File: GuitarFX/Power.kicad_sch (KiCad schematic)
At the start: 20 parts, among them J201 Jack-DC, U3 NCP718xSN500, U4 NCP1117-3.3_SOT223

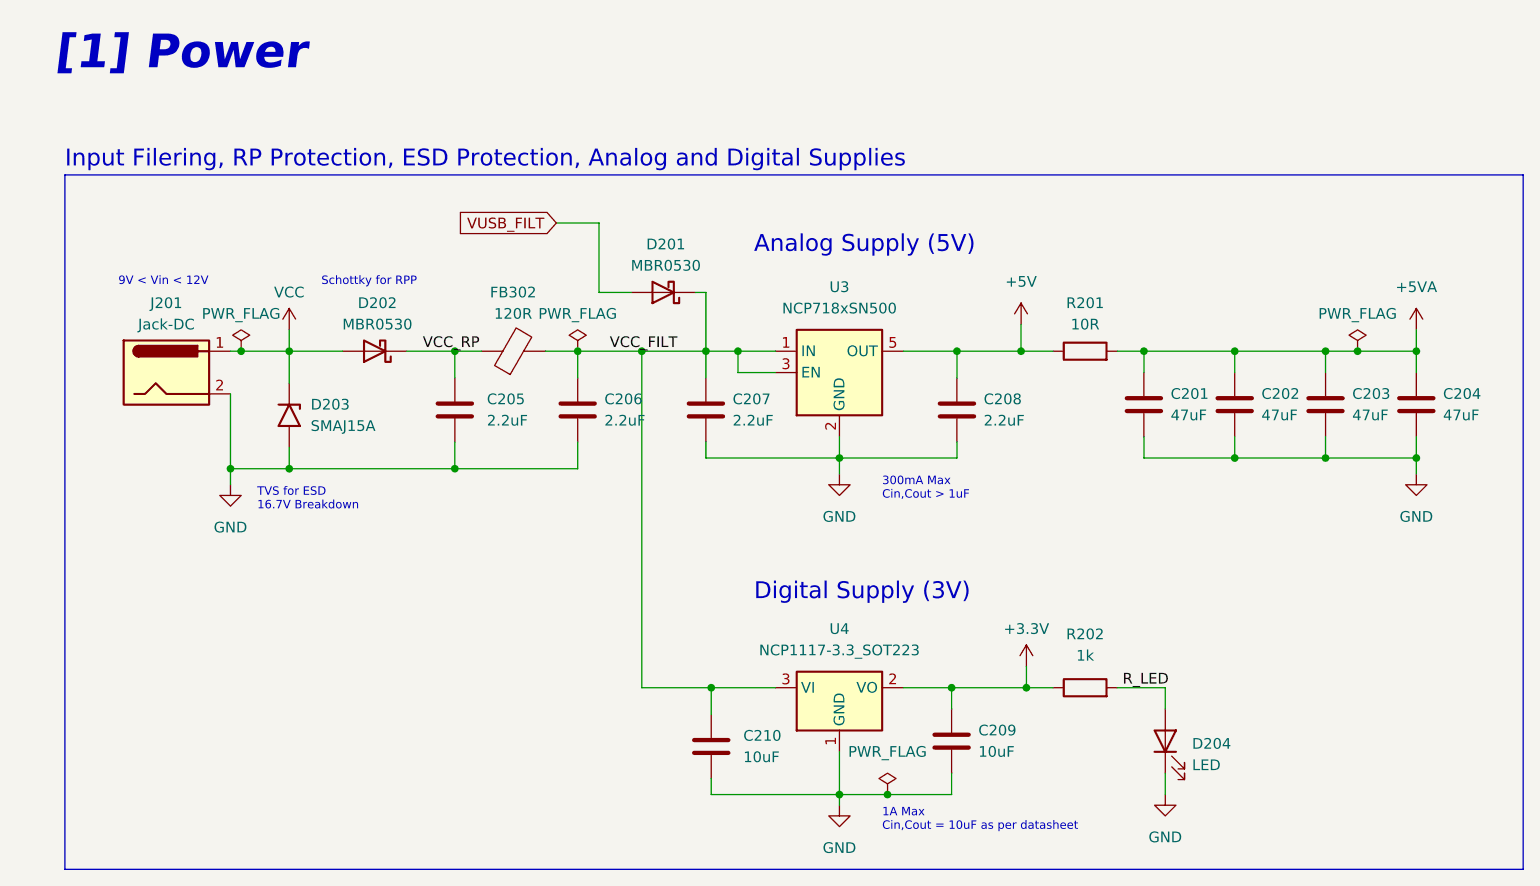
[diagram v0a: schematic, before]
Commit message: Assigned all footprints
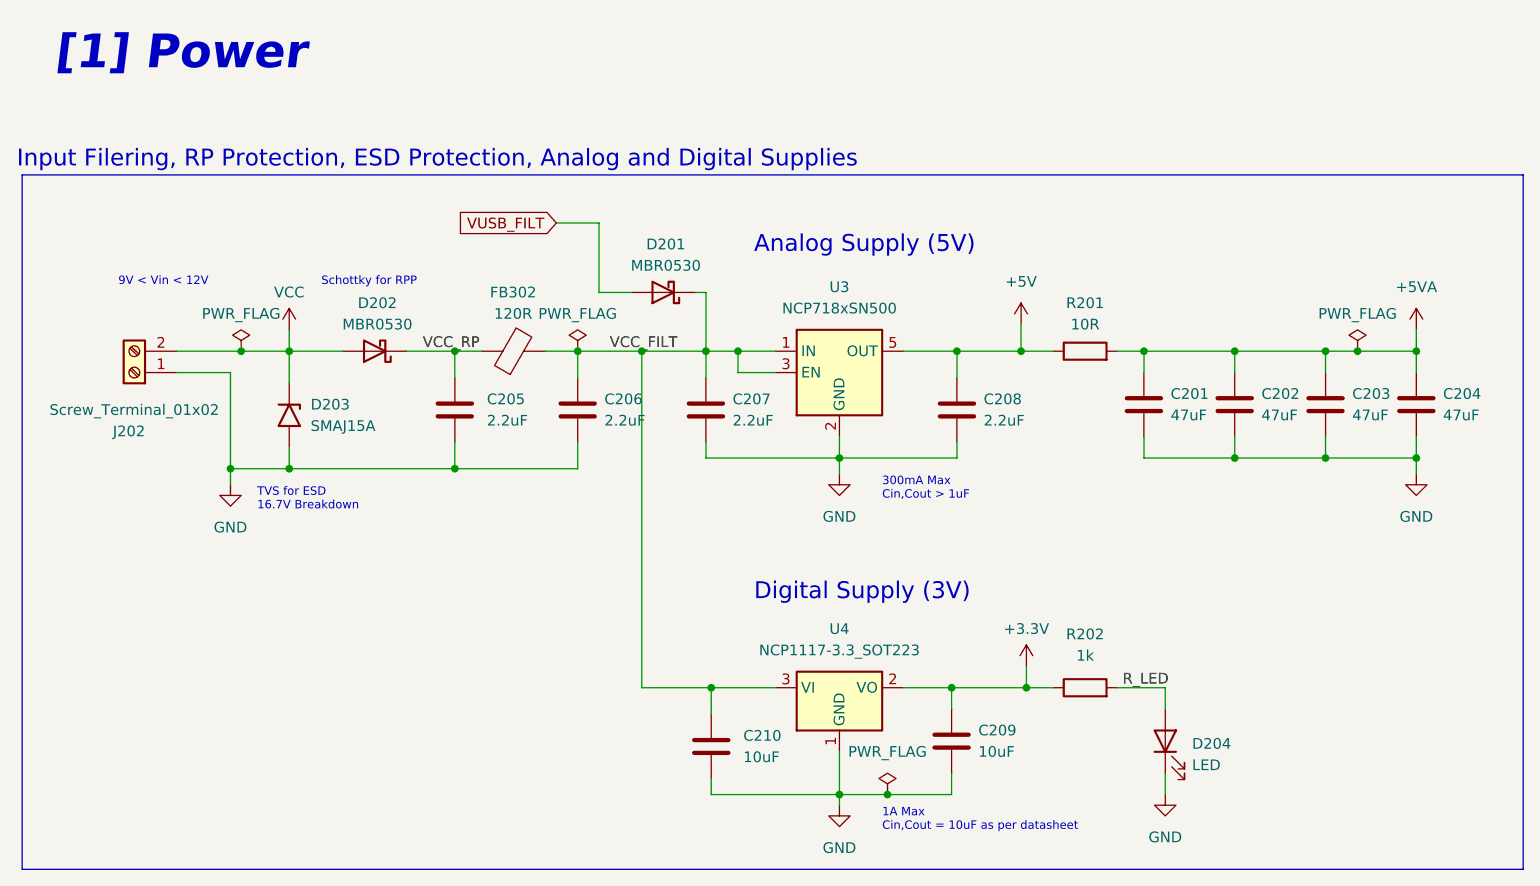
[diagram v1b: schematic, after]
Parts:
- removed J201: Jack-DC, symbol Connector:Jack-DC
- added J202: Screw_Terminal_01x02, TerminalBlock_Phoenix:TerminalBlock_Phoenix_MPT-0,5-2-2.54_1x02_P2.54mm_Horizontal, symbol Connector:Screw_Terminal_01x02
- FB302: footprint (none) -> Inductor_SMD:L_0603_1608Metric
- R201: footprint (none) -> TerminalBlock_Phoenix:TerminalBlock_Phoenix_MPT-0,5-6-2.54_1x06_P2.54mm_Horizontal
- R202: footprint (none) -> TerminalBlock_Phoenix:TerminalBlock_Phoenix_MPT-0,5-4-2.54_1x04_P2.54mm_Horizontal
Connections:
- net GND: now also J202.1 (Pin_1)
- net VCC: now also J202.2 (Pin_2)
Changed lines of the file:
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@@
-    (stroke (width 0) (type default))
-  )
-  (wire (pts (xy 60.96 62.865) (xy 62.23 62.865))
     (stroke (width 0) (type default))
   )
@@
     (stroke (width 0) (type default))
   )
+  (wire (pts (xy 54.61 62.865) (xy 62.23 62.865))
+    (stroke (width 0) (type default))
+  )
   (wire (pts (xy 118.11 115.57) (xy 133.35 115.57))
     (stroke (width 0) (type default))
@@
     (stroke (width 0) (type default))
   )
-  (wire (pts (xy 60.96 67.945) (xy 60.96 76.835))
+  (wire (pts (xy 60.96 65.405) (xy 60.96 76.835))
     (stroke (width 0) (type default))
   )
@@
     (stroke (width 0) (type default))
   )
+  (wire (pts (xy 54.61 65.405) (xy 60.96 65.405))
+    (stroke (width 0) (type default))
+  )
   (wire (pts (xy 191.135 73.025) (xy 191.135 75.565))
     (stroke (width 0) (type default))
@@
     (stroke (width 0) (type default))
   )
-  (rectangle (start 41.275 41.91) (end 214.63 124.46)
+  (rectangle (start 36.195 41.91) (end 214.63 124.46)
     (stroke (width 0) (type default))
     (fill (type none))
@@
   )
   (text "Input Filering, RP Protection, ESD Protection, Analog and Digital Supplies"
-    (at 41.275 41.275 0)
+    (at 35.56 41.275 0)
     (effects (font (size 2 2)) (justify left bottom))
   )
@@
       (effects (font (size 1.27 1.27)))
     )
-    (property "Footprint" "" (at 162.56 104.648 90)
+    (property "Footprint" "TerminalBlock_Phoenix:TerminalBlock_Phoenix_MPT-0,5-4-2.54_1x04_P2.54mm_Horizontal" (at 162.56 104.648 90)
       (effects (font (size 1.27 1.27)) hide)
     )
@@
       (effects (font (size 1.27 1.27)))
     )
-    (property "Footprint" "" (at 162.56 64.643 90)
+    (property "Footprint" "TerminalBlock_Phoenix:TerminalBlock_Phoenix_MPT-0,5-6-2.54_1x06_P2.54mm_Horizontal" (at 162.56 64.643 90)
       (effects (font (size 1.27 1.27)) hide)
     )
@@
         (path "/4ab4bfc6-98ca-4cb1-8273-436b96035b51/171d6b95-1f9c-4c9d-954a-bc461d0cb77a"
           (reference "R201") (unit 1)
-        )
-      )
-    )
-  )
-  (symbol (lib_id "Connector:Jack-DC") (at 53.34 65.405 0) (unit 1)
-    (in_bom yes) (on_board yes) (dnp no) (fields_autoplaced)
-    (property "Reference" "J201" (at 53.34 57.15 0)
-      (effects (font (size 1.27 1.27)))
-    )
-    (property "Value" "Jack-DC" (at 53.34 59.69 0)
-      (effects (font (size 1.27 1.27)))
-    )
-    (property "Footprint" "" (at 54.61 66.421 0)
-      (effects (font (size 1.27 1.27)) hide)
-    )
-    (property "Datasheet" "~" (at 54.61 66.421 0)
-      (effects (font (size 1.27 1.27)) hide)
-    )
-    (pin "1")
-    (pin "2")
-    (instances
-      (project "GuitarFX"
-        (path "/4ab4bfc6-98ca-4cb1-8273-436b96035b51/171d6b95-1f9c-4c9d-954a-bc461d0cb77a"
-          (reference "J201") (unit 1)
         )
       )
@@
       (effects (font (size 1.27 1.27)))
     )
-    (property "Footprint" "" (at 94.615 64.643 90)
+    (property "Footprint" "Inductor_SMD:L_0603_1608Metric" (at 94.615 64.643 90)
       (effects (font (size 1.27 1.27)) hide)
     )
@@
         )
       )
+    )
+  )
+  (symbol (lib_id "Connector:Screw_Terminal_01x02") (at 49.53 65.405 180) (unit 1)
+    (in_bom yes) (on_board yes) (dnp no)
+    (property "Reference" "J202" (at 48.895 72.39 0)
+      (effects (font (size 1.27 1.27)))
+    )
+    (property "Value" "Screw_Terminal_01x02" (at 49.53 69.85 0)
+      (effects (font (size 1.27 1.27)))
+    )
+    (property "Footprint" "TerminalBlock_Phoenix:TerminalBlock_Phoenix_MPT-0,5-2-2.54_1x02_P2.54mm_Horizontal" (at 49.53 65.405 0)
+      (effects (font (size 1.27 1.27)) hide)
+    )
+    (property "Datasheet" "~" (at 49.53 65.405 0)
+      (effects (font (size 1.27 1.27)) hide)
+    )
+    (pin "1")
+    (pin "2")
+    (instances
+      (project "GuitarFX"
+        (path "/4ab4bfc6-98ca-4cb1-8273-436b96035b51/171d6b95-1f9c-4c9d-954a-bc461d0cb77a"
+          (reference "J202") (unit 1)
+        )
+      )
